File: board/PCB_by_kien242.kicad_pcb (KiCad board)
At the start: 2 copper layers, 61 x 63.5 mm, 27 parts, among them J1 VIN, J2 , J4 TC1, J6 SSR1, J7 SSR2, J8 SSR3, Q4 IRLR2905Z, Q5 IRLR2905Z, Q6 IRLR2905Z, Q7 2N3904, Q8 2N3904, U2 YAAJ_DCDC_StepDown_LM2596, U4 MAX31855KASA, U5 ESP32-WROOM-32, U6 CH340G, Y1 12mhz

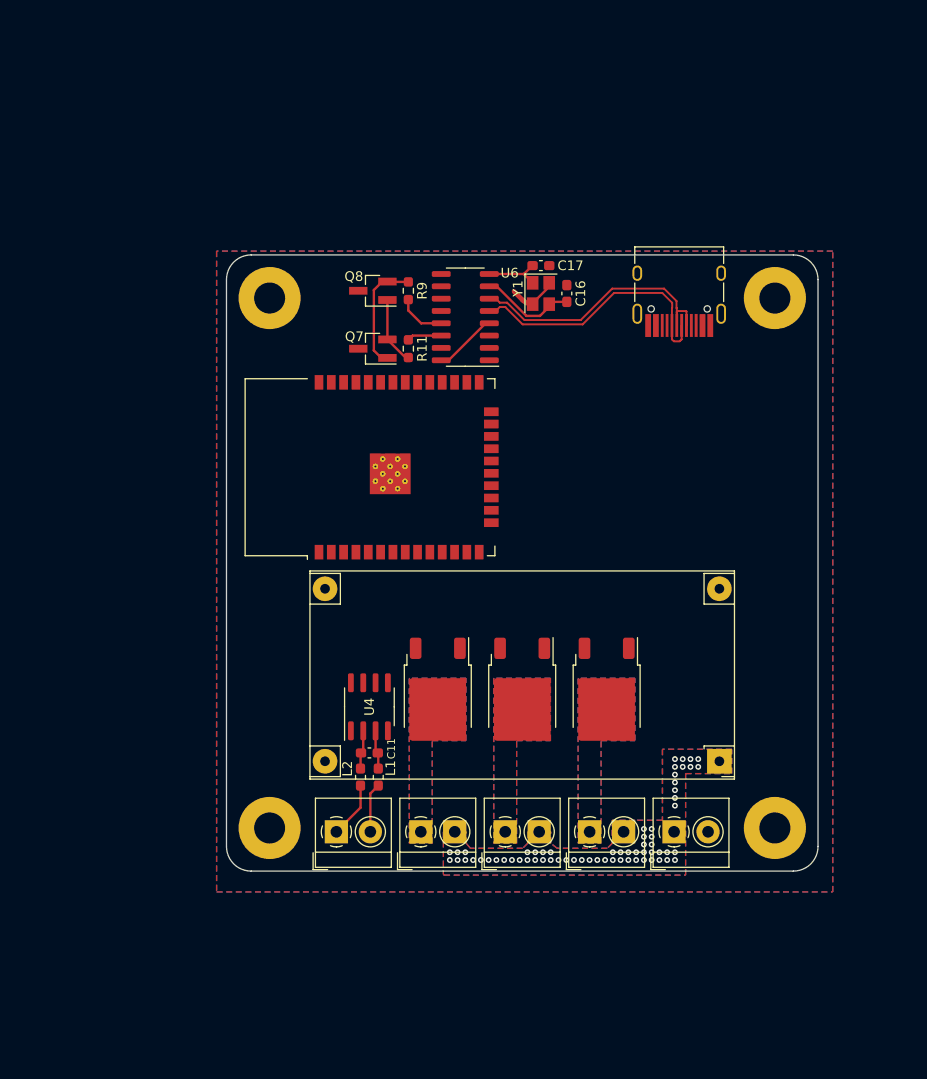
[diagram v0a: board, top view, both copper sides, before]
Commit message: Update
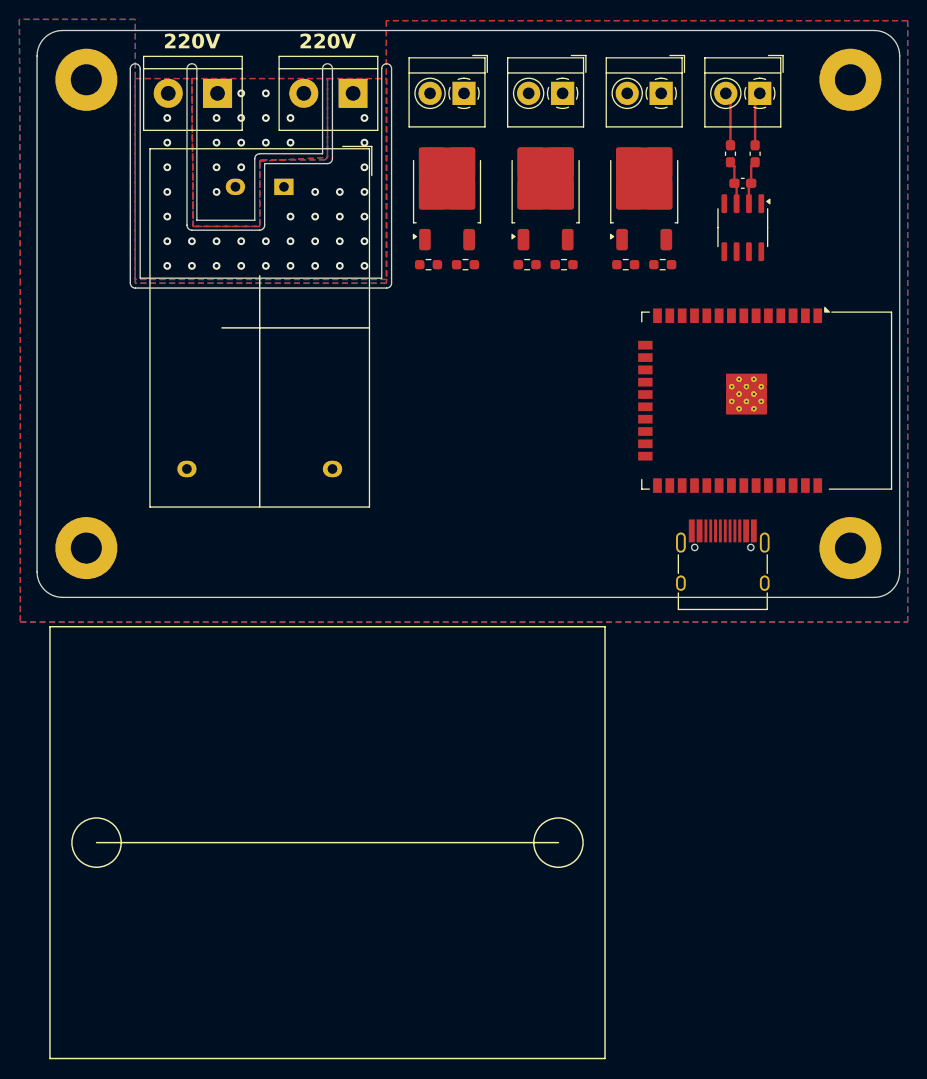
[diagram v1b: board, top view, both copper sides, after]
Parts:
- removed C16, C17: 22, Capacitor_SMD:C_0603_1608Metric_Pad1.08x0.95mm_HandSolder
- removed Q7, Q8: 2N3904, Package_TO_SOT_SMD:SOT-23_Handsoldering
- removed R11, R9: 22r, Resistor_SMD:R_0603_1608Metric_Pad0.98x0.95mm_HandSolder
- removed U2: YAAJ_DCDC_StepDown_LM2596, TerminalBlock_KF301:YAAJ_DCDC_StepDown_LM2596
- removed U6: CH340G, Package_SO:SOIC-16_3.9x9.9mm_P1.27mm
- removed Y1: 12mhz, Crystal:Crystal_SMD_3225-4Pin_3.2x2.5mm
- added J3: VIN, TerminalBlock:TerminalBlock_bornier-2_P5.08mm, F.Cu at (66.1, 29.5)
- added PS1: HLK-PM05, Converter_ACDC:Converter_ACDC_Hi-Link_HLK-PMxx, F.Cu at (73.0, 39.1)
- added R19: R_Small, Resistor_SMD:R_0603_1608Metric_Pad0.98x0.95mm_HandSolder, F.Cu at (108.2, 47.1)
- added R20: R_Small, Resistor_SMD:R_0603_1608Metric_Pad0.98x0.95mm_HandSolder, F.Cu at (98.0, 47.1)
- added R21: ??, Resistor_SMD:R_0603_1608Metric_Pad0.98x0.95mm_HandSolder, F.Cu at (87.9, 47.1)
- added R22: 10k, Resistor_SMD:R_0603_1608Metric_Pad0.98x0.95mm_HandSolder, F.Cu at (112.0, 47.1)
- added R23: 10k, Resistor_SMD:R_0603_1608Metric_Pad0.98x0.95mm_HandSolder, F.Cu at (101.9, 47.1)
- added R24: 10k, Resistor_SMD:R_0603_1608Metric_Pad0.98x0.95mm_HandSolder, F.Cu at (91.7, 47.1)
- J1: footprint TerminalBlock_4Ucon:TerminalBlock_4Ucon_1x02_P3.50mm_Horizontal -> TerminalBlock:TerminalBlock_bornier-2_P5.08mm
- moved J4 87.7 mm to (122.0, 29.5), turned to 180 degrees
- moved J1 83.0 mm to (80.1, 29.5), turned to 180 degrees
- moved J6 80.0 mm to (111.9, 29.5), turned to 180 degrees
- moved J8 77.2 mm to (91.5, 29.5), turned to 180 degrees
- moved H4 76.6 mm to (52.6, 76.3)
- moved J7 76.3 mm to (101.7, 29.5), turned to 180 degrees
- moved L2 76.0 mm to (121.5, 35.7), turned to 90 degrees
- moved H1 74.4 mm to (52.6, 28.1)
- moved L1 73.8 mm to (119.0, 35.7), turned to 90 degrees
- moved C11 70.2 mm to (120.3, 38.7), turned to 0 degrees
- moved H3 66.4 mm to (131.4, 76.3)
- moved H2 63.9 mm to (131.4, 28.1)
- moved U4 62.6 mm to (120.3, 43.3), turned to -90 degrees
- moved Q4 56.4 mm to (110.1, 39.5), turned to 90 degrees
- moved Q6 54.7 mm to (89.8, 39.5), turned to 90 degrees
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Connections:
- J1 pad 1: V_SSR -> Net-(J1-Pin_1)
- J1 pad 2: GND -> Net-(J1-Pin_2)
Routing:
- net D+: track 27.9 -> 0.00 mm
- net D-: track 27.2 -> 0.00 mm
- net Net-(Q7-B): track 11.9 -> 0.00 mm
- net Net-(U6-XI): track 10.0 -> 0.00 mm
- net Net-(Q7-E): track 7.00 -> 0.00 mm
- net +3.3V: track 6.53 -> 0.00 mm
- net Net-(U6-XO): track 6.10 -> 0.00 mm
- net GND: track 5.26 -> 0.00 mm
- net DTR: track 5.06 -> 0.00 mm
- net RTS: track 3.57 -> 0.00 mm
- net Net-(U4-T+): track 4.00 -> 4.53 mm
- net Net-(U4-T-): track 4.00 -> 4.53 mm
- net V_SSR: vias 65 -> 0
- net Net-(J1-Pin_2): vias 0 -> 13
- net Net-(J1-Pin_1): vias 0 -> 33
- added copper zone on B.Cu, net Net-(J1-Pin_1)
- added copper zone on F.Cu, net Net-(J1-Pin_1)
- added copper zone on B.Cu, net Net-(J1-Pin_2)
- added copper zone on F.Cu, net Net-(J1-Pin_2)
- removed copper zone on B.Cu, net Net-(J6-Pin_1)
- removed copper zone on F.Cu, net Net-(J6-Pin_1)
- removed copper zone on B.Cu, net Net-(J7-Pin_1)
- removed copper zone on F.Cu, net Net-(J7-Pin_1)
- removed copper zone on B.Cu, net Net-(J8-Pin_1)
- removed copper zone on F.Cu, net Net-(J8-Pin_1)
- removed copper zone on B.Cu, net V_SSR
- removed copper zone on F.Cu, net V_SSR
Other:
- board size 61 x 63.5 mm -> 88.9 x 58.4 mm
- board text added: "220V"
